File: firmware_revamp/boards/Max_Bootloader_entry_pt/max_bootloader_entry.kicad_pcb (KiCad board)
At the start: 2 copper layers, 58.3 x 109.3 mm, 37 parts, among them J2 CONN_02X03, J3 CONN_01X03, J4 Conn_01x10, J5 Conn_01x10, U1 ATMEGA16M1, U2 MIC5205-3.3YM5, U3 FT231XS, U4 MCP2561-E_SN, U5 USB_MicroB, Y1 Crystal_SMD

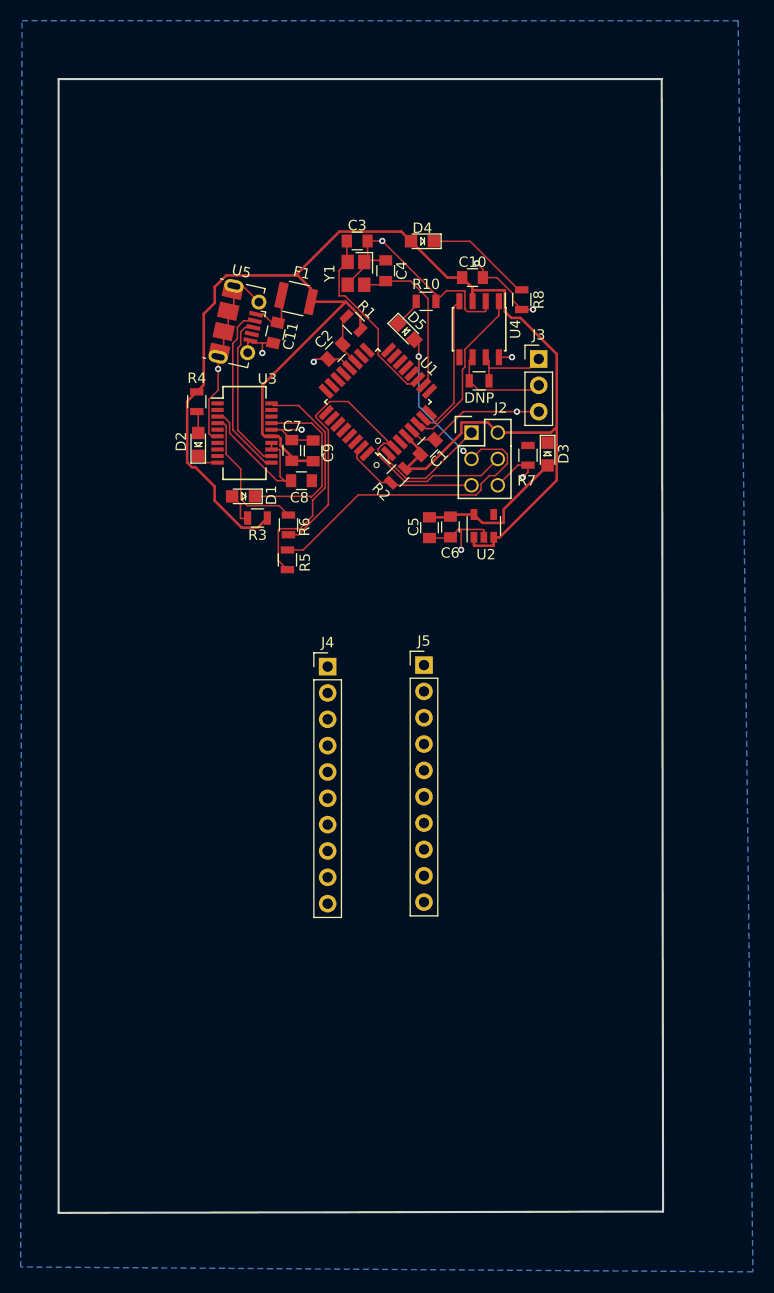
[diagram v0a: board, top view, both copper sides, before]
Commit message: What I have so far on bootloader board
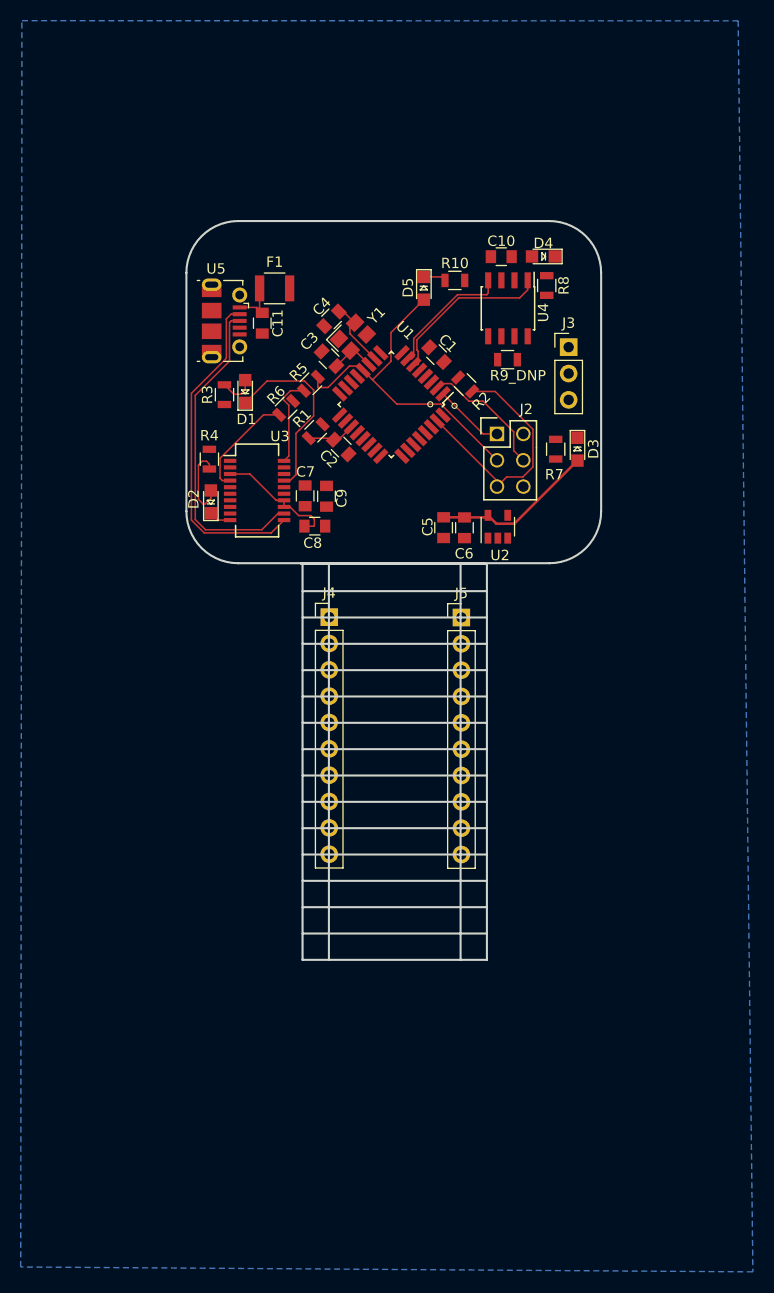
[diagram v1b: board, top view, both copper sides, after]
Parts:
- moved R5 17.1 mm to (57.9, 74.7), turned to 45 degrees
- moved R3 12.3 mm to (49.5, 75.7), turned to 270 degrees
- moved D4 11.8 mm to (80.3, 62.4)
- moved C3 11.7 mm to (59.6, 72.3), turned to 135 degrees
- moved R6 11.3 mm to (55.5, 77.0), turned to 45 degrees
- moved R1 11.0 mm to (58.3, 79.3), turned to 225 degrees
- moved R2 10.9 mm to (72.7, 74.7), turned to 315 degrees
- moved D1 10.1 mm to (51.5, 75.4), turned to 90 degrees
- moved C2 9.21 mm to (60.8, 80.8), turned to 315 degrees
- moved C1 8.96 mm to (70.0, 71.9), turned to 135 degrees
- moved C4 6.99 mm to (59.9, 68.4), turned to 225 degrees
- moved Y1 6.12 mm to (61.9, 70.1), turned to 45 degrees
- moved J5 5.84 mm to (72.4, 97.2)
- moved D2 5.67 mm to (48.2, 86.1)
- moved R4 5.67 mm to (48.1, 81.9)
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- renumbered DNP to R9_DNP
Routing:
- net +5V: track 151.8 -> 0.00 mm
- net GND: track 95.2 -> 0.00 mm, vias 11 -> 0
- net /MOSI: track 40.2 -> 12.6 mm
- net /USBD-: track 15.3 -> 31.0 mm
- net /USBD+: track 17.1 -> 32.2 mm
- net Net-(R5-Pad1): track 23.0 -> 8.76 mm
- net Net-(C3-Pad1): track 18.4 -> 4.39 mm
- net /SCK: track 45.7 -> 32.7 mm, vias 2 -> 0
- net /RESET: track 13.3 -> 24.0 mm
- net Net-(D4-Pad1): track 10.4 -> 0.00 mm
- net /CAN_-: track 9.66 -> 0.00 mm
- net Net-(C4-Pad1): track 15.5 -> 6.68 mm
- net /CAN_+: track 7.57 -> 0.00 mm
- net Net-(D2-Pad2): track 2.13 -> 8.01 mm
- net /MISO: track 11.2 -> 6.80 mm
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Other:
- board size 58.3 x 109.3 mm -> 40 x 71.3 mm
